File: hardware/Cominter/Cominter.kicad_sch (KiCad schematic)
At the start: 8 parts, among them U1 MCP6002-xP

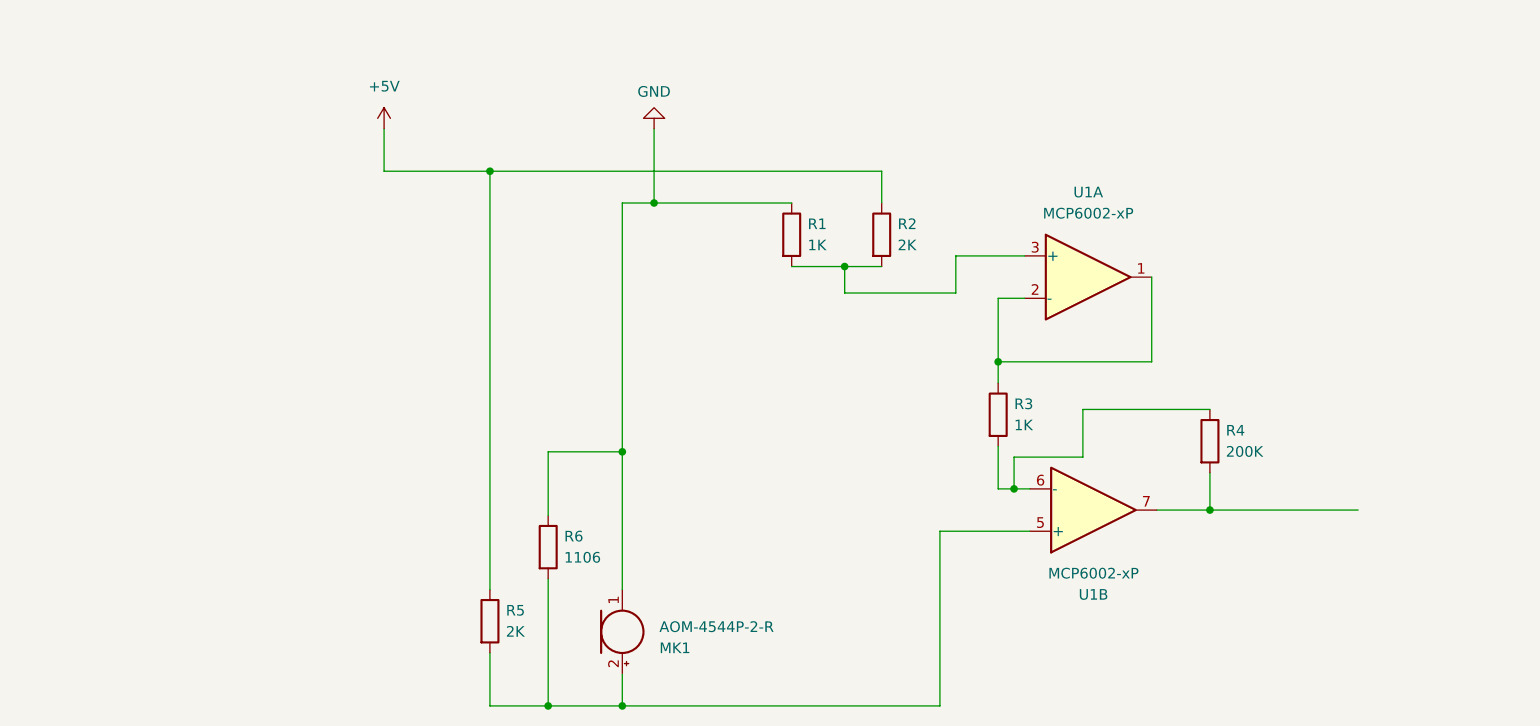
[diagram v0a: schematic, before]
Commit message: WIP
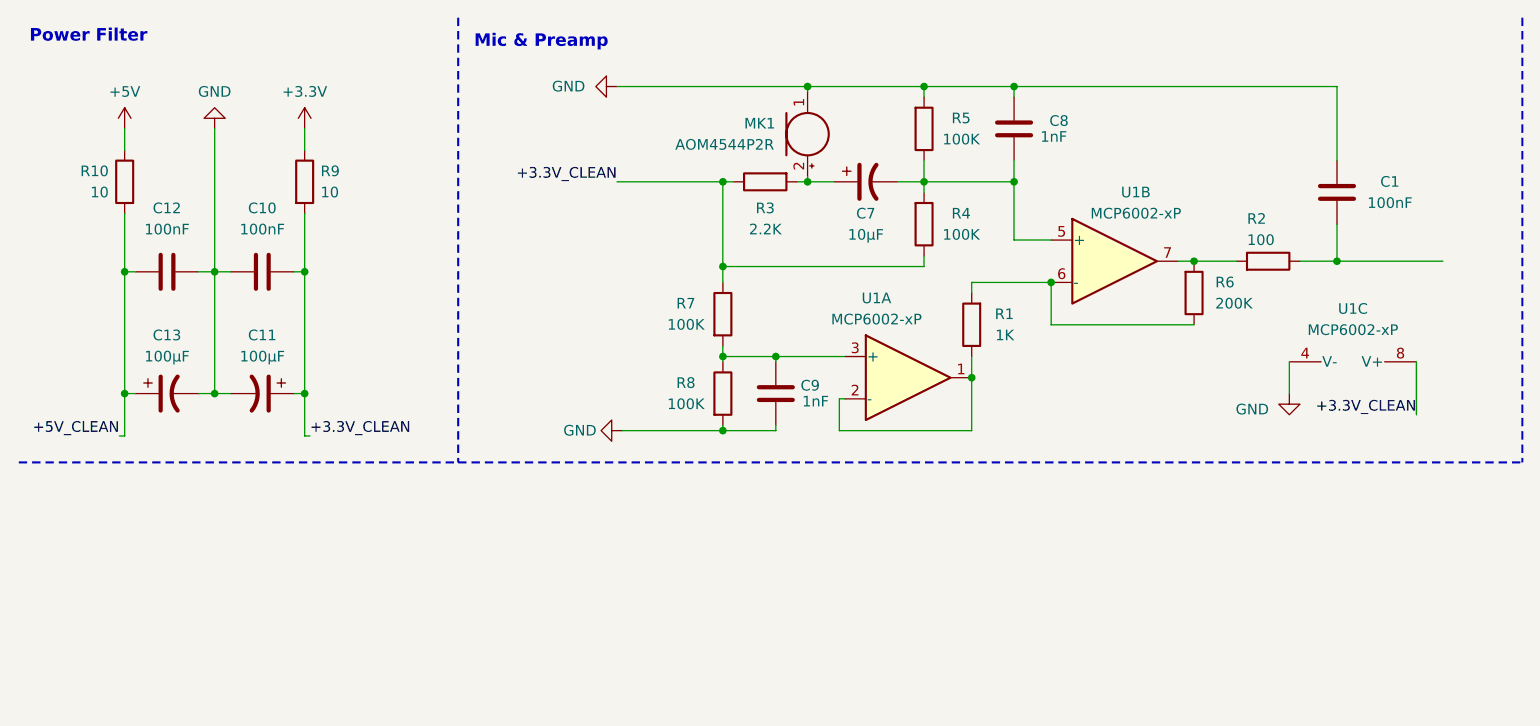
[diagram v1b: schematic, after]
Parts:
- added C1, C10, C12: 100nF, symbol Device:C
- added C11, C13: 100µF, symbol Device:C_Polarized_US
- added C7: 10µF, symbol Device:C_Polarized_US
- added C8, C9: 1nF, symbol Device:C
- added R10, R9: 10, symbol Device:R
- added R7, R8: 100K, symbol Device:R
- added unit 3 of U1
- MK1: value AOM-4544P-2-R -> AOM4544P2R
- R2: value 2K -> 100
- R3: value 1K -> 2.2K
- R4: value 200K -> 100K
- R5: value 2K -> 100K
- R6: value 1106 -> 200K
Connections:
- net +5V: now also R10.1; no longer R2.1, R5.1
- net GND: now also R5.2, C1.1, C10.1, C11.2, C12.1, C13.2, C8.1, C9.1, R8.2, U1.4 (V-); no longer R1.1, R6.1
- net at R4.2: now also R5.1, U1.5 (+), C7.2, C8.2; no longer U1.7
- net at U1.1, U1.2 (-): now also R1.1; no longer R3.1
- new net: C7.1, MK1.2 (+), R3.2
- new net: R1.2, R6.1, U1.6 (-)
- new net: C1.2, R2.1
- new net: C9.2, R7.2, R8.1, U1.3 (+)
- new net: R2.2, R6.2, U1.7
- new net +3.3V: R9.1
- new net +3.3V_CLEAN: C10.2, C11.1, R3.1, R4.1, R7.1, R9.2, U1.8 (V+)
- new net +5V_CLEAN: C12.2, C13.1, R10.2
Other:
- note added: "Mic & Preamp"
- note added: "Power Filter"
- moved on the sheet: U1A, U1B
